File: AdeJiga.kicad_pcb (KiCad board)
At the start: 2 copper layers, 72 x 72 mm, 33 parts, among them J1 Screw_Terminal_01x03, J10 Conn_01x02_Pin, J11 Conn_01x02_Pin, J2 Screw_Terminal_01x02, J3 Screw_Terminal_01x03, J4 Conn_01x05_Pin, J5 Conn_01x02_Pin, J6 Conn_01x03_Pin, J7 Conn_01x02_Pin, J8 Conn_01x03_Pin, J9 Conn_01x04_Pin, K1 JJM1C_relay, K2 JJM1C_relay, M1 DC-DC-STEP-DOWN-LM2596, Q1 TIP127, Q3 TIP127, U2 ESP32-WROOM-32, U4 AMS1117

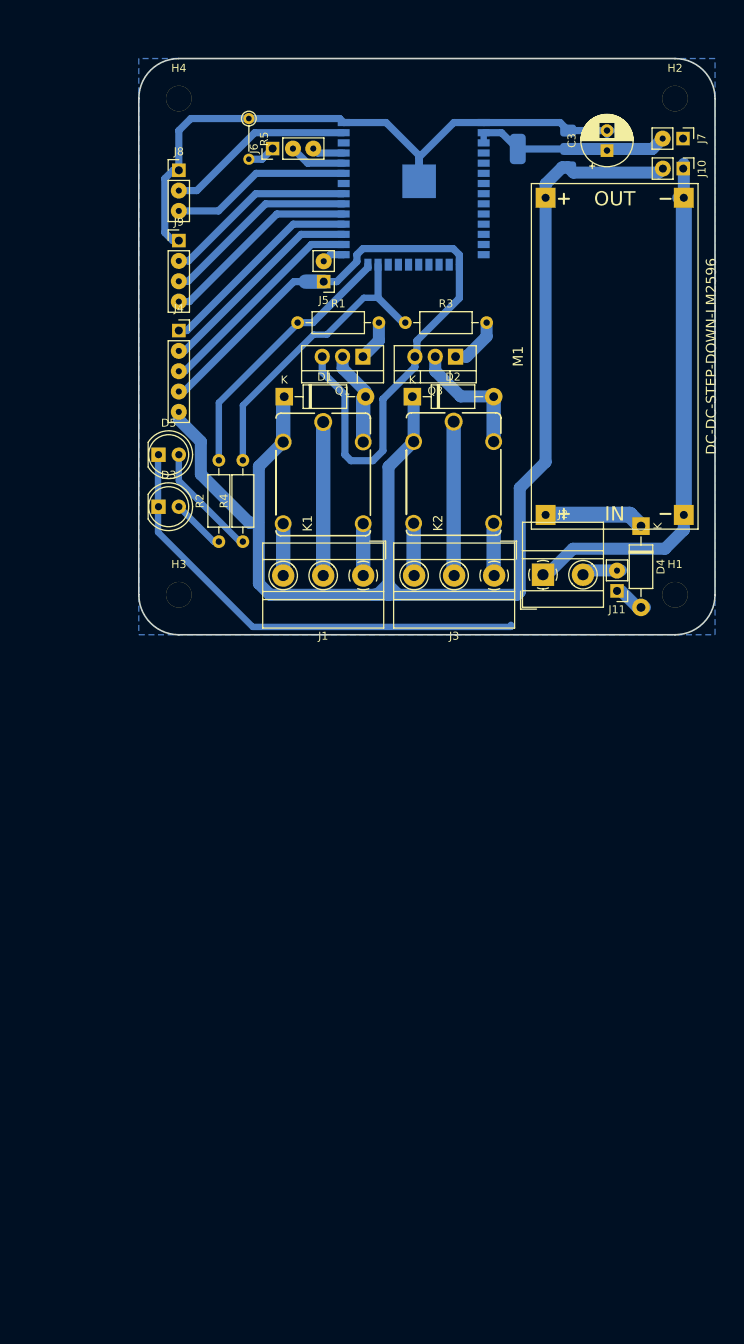
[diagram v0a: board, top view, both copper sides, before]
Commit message: 3 reles na jiga
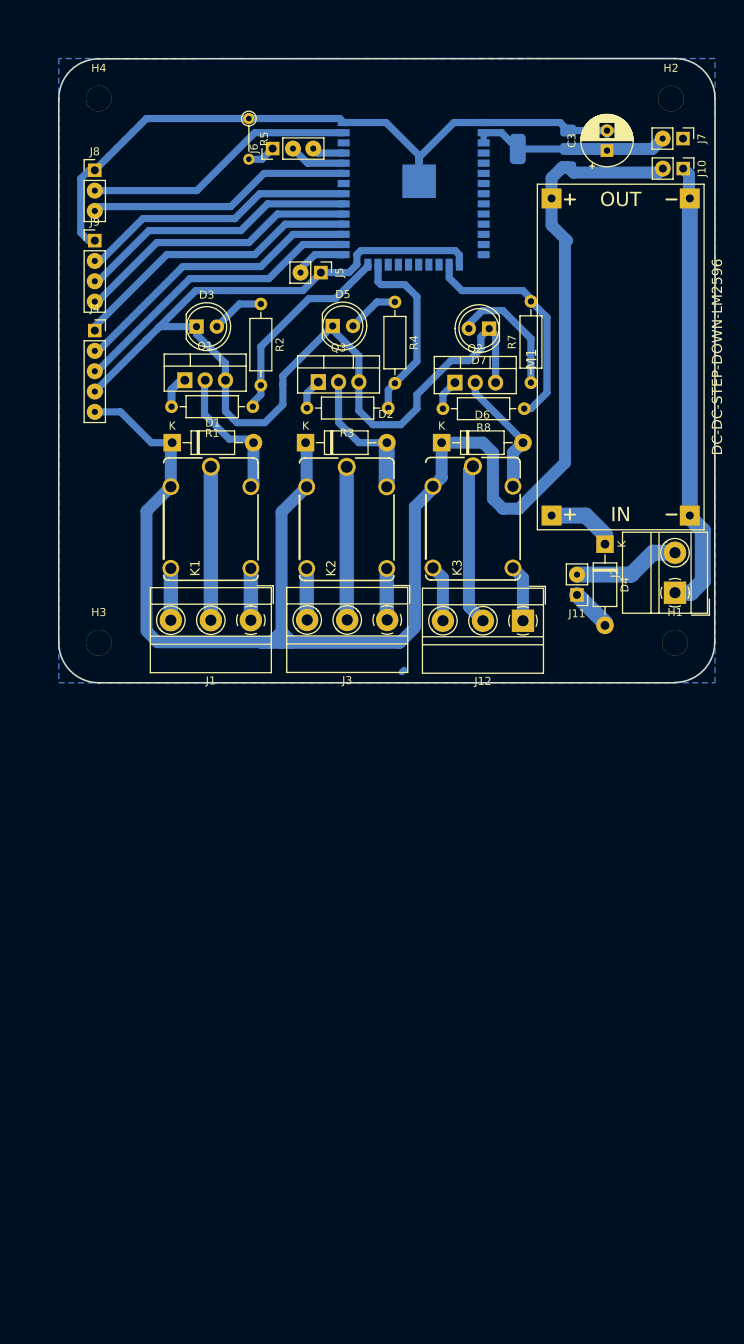
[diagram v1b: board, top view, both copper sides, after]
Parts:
- added D6: 1N4007, Diode_THT:D_DO-41_SOD81_P10.16mm_Horizontal, F.Cu at (159.8, 71.0)
- added D7: LED, LED_THT:LED_D5.0mm_Clear, F.Cu at (165.8, 56.8)
- added J12: Screw_Terminal_01x03, TerminalBlock_MetzConnect:TerminalBlock_MetzConnect_Type011_RT05503HBWC_1x03_P5.00mm_Horizontal, F.Cu at (170.0, 93.2)
- added K3: JJM1C_relay, Benzlab:JJM1C_relay, F.Cu at (163.8, 80.5)
- added Q2: TIP127, Package_TO_SOT_THT:TO-220-3_Vertical, F.Cu at (161.5, 63.5)
- added R7: 220, Resistor_THT:R_Axial_DIN0207_L6.3mm_D2.5mm_P10.16mm_Horizontal, F.Cu at (171.0, 63.5)
- added R8: 3.3k, Resistor_THT:R_Axial_DIN0207_L6.3mm_D2.5mm_P10.16mm_Horizontal, F.Cu at (170.2, 66.8)
- moved R4 35.5 mm to (154.0, 53.4), turned to -90 degrees
- moved R2 30.2 mm to (137.2, 53.7), turned to -90 degrees
- moved D5 27.1 mm to (146.2, 56.4)
- moved D3 23.0 mm to (129.2, 56.5)
- moved Q1 22.4 mm to (127.8, 63.2), turned to 0 degrees
- moved Q3 17.5 mm to (144.4, 63.4), turned to 0 degrees
- moved J2 16.7 mm to (189.0, 89.8), turned to 90 degrees
- moved D1 15.1 mm to (126.2, 71.0)
- moved J1 15.1 mm to (136.0, 93.2)
- moved K1 15.1 mm to (131.0, 80.5)
- moved D2 14.5 mm to (142.8, 71.0)
- moved K2 14.5 mm to (148.0, 80.6)
- moved J3 14.5 mm to (153.0, 93.2)
- moved R1 11.9 mm to (136.2, 66.5), turned to 180 degrees
- moved H3 11.7 mm to (117.0, 96.0)
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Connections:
- net GPIO16 renamed REL1
- net GPIO17 renamed REL2
- U2 pad 16: unconnected-(U2-IO13-Pad16) -> REL3
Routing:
- net REL3: track 0.00 -> 29.2 mm
- net +5V: track 175.3 -> 202.5 mm
- net Net-(J12-Pin_2): track 0.00 -> 20.2 mm
- net Net-(D7-A): track 0.00 -> 16.0 mm
- net Ativa_Relé_3: track 0.00 -> 15.9 mm
- net REL2: track 38.2 -> 23.2 mm
- net GND: track 297.3 -> 283.2 mm
- net GPIOC: track 26.1 -> 36.9 mm
- net GPIOE: track 24.6 -> 35.1 mm
- net GPIOA: track 27.2 -> 37.7 mm
- net GPIOG: track 23.6 -> 34.1 mm
- net GPIOD: track 25.1 -> 35.6 mm
- net GPIOB: track 26.6 -> 37.1 mm
- net GPIOH: track 22.5 -> 33.0 mm
- net GPIOF: track 24.1 -> 34.6 mm
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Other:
- board size 72 x 72 mm -> 82 x 78 mm

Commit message: Versão 3 consolidada, placa fabricada
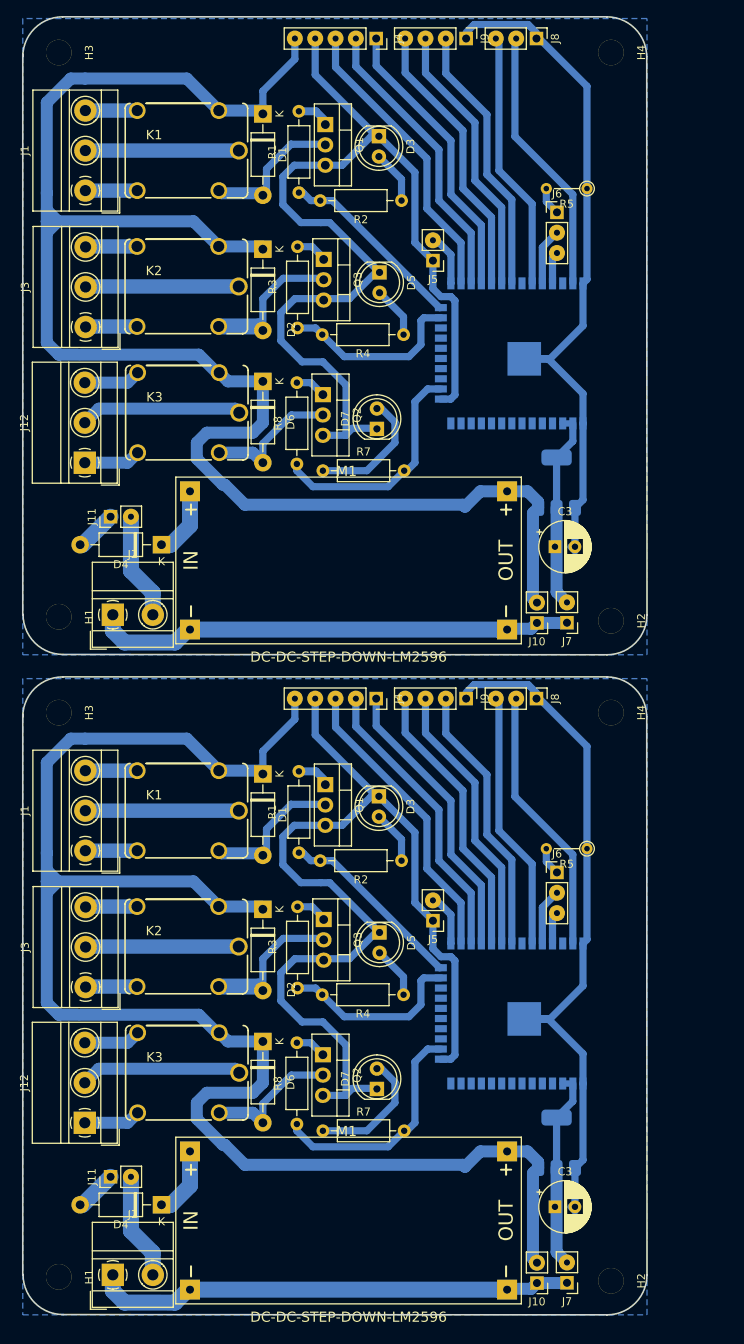
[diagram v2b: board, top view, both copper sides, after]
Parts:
- added C3: 220uF, Capacitor_THT:CP_Radial_D6.3mm_P2.50mm, F.Cu at (174.0, 166.5)
- added D1: 1N4007, Diode_THT:D_DO-41_SOD81_P10.16mm_Horizontal, F.Cu at (137.5, 112.4)
- added D2: 1N4007, Diode_THT:D_DO-41_SOD81_P10.16mm_Horizontal, F.Cu at (137.5, 129.3)
- added D3: LED, LED_THT:LED_D5.0mm_Clear, F.Cu at (152.0, 115.2)
- added D4: 1N4007, Diode_THT:D_DO-41_SOD81_P10.16mm_Horizontal, F.Cu at (124.8, 166.2)
- added D5: LED, LED_THT:LED_D5.0mm_Clear, F.Cu at (152.1, 132.2)
- added D6: 1N4007, Diode_THT:D_DO-41_SOD81_P10.16mm_Horizontal, F.Cu at (137.5, 145.8)
- added D7: LED, LED_THT:LED_D5.0mm_Clear, F.Cu at (151.8, 151.8)
- added H1: MountingHole, MountingHole:MountingHole_3.2mm_M3_DIN965, F.Cu at (112.0, 175.2)
- added H2: MountingHole, MountingHole:MountingHole_3.2mm_M3_DIN965, F.Cu at (181.0, 175.7)
- added H3: MountingHole, MountingHole:MountingHole_3.2mm_M3_DIN965, F.Cu at (112.0, 104.7)
- added H4: MountingHole, MountingHole:MountingHole_3.2mm_M3_DIN965, F.Cu at (181.0, 104.7)
- added J1: Screw_Terminal_01x03, TerminalBlock_MetzConnect:TerminalBlock_MetzConnect_Type011_RT05503HBWC_1x03_P5.00mm_Horizontal, F.Cu at (115.3, 122.0)
- added J10: Conn_01x02_Pin, Connector_PinHeader_2.54mm:PinHeader_1x02_P2.54mm_Vertical, F.Cu at (171.8, 176.0)
- added J11: Conn_01x02_Pin, Connector_PinHeader_2.54mm:PinHeader_1x02_P2.54mm_Vertical, F.Cu at (118.5, 162.7)
- added J12: Screw_Terminal_01x03, TerminalBlock_MetzConnect:TerminalBlock_MetzConnect_Type011_RT05503HBWC_1x03_P5.00mm_Horizontal, F.Cu at (115.2, 156.0)
- added J2: Screw_Terminal_01x02, TerminalBlock_MetzConnect:TerminalBlock_MetzConnect_Type011_RT05502HBWC_1x02_P5.00mm_Horizontal, F.Cu at (118.8, 175.0)
- added J3: Screw_Terminal_01x03, TerminalBlock_MetzConnect:TerminalBlock_MetzConnect_Type011_RT05503HBWC_1x03_P5.00mm_Horizontal, F.Cu at (115.3, 139.0)
- added J4: Conn_01x05_Pin, Connector_PinSocket_2.54mm:PinSocket_1x05_P2.54mm_Vertical, F.Cu at (151.7, 103.0)
- added J5: Conn_01x02_Pin, Connector_PinHeader_2.54mm:PinHeader_1x02_P2.54mm_Vertical, F.Cu at (158.8, 130.7)
- added J6: Conn_01x03_Pin, Connector_PinHeader_2.54mm:PinHeader_1x03_P2.54mm_Vertical, F.Cu at (174.2, 124.7)
- added J7: Conn_01x02_Pin, Connector_PinHeader_2.54mm:PinHeader_1x02_P2.54mm_Vertical, F.Cu at (175.5, 176.0)
- added J8: Conn_01x03_Pin, Connector_PinHeader_2.54mm:PinHeader_1x03_P2.54mm_Vertical, F.Cu at (171.7, 103.0)
- added J9: Conn_01x04_Pin, Connector_PinHeader_2.54mm:PinHeader_1x04_P2.54mm_Vertical, F.Cu at (162.9, 103.0)
- added K1: JJM1C_relay, Benzlab:JJM1C_relay, F.Cu at (128.0, 117.0)
- added K2: JJM1C_relay, Benzlab:JJM1C_relay, F.Cu at (127.9, 134.0)
- added K3: JJM1C_relay, Benzlab:JJM1C_relay, F.Cu at (128.0, 149.7)
- added M1: DC-DC-STEP-DOWN-LM2596, Benzlab:DC-DC-STEP-DOWN-LM2596, F.Cu at (148.2, 168.2)
- added Q1: TIP127, Package_TO_SOT_THT:TO-220-3_Vertical, F.Cu at (145.3, 113.7)
- added Q2: TIP127, Package_TO_SOT_THT:TO-220-3_Vertical, F.Cu at (145.0, 147.5)
- added Q3: TIP127, Package_TO_SOT_THT:TO-220-3_Vertical, F.Cu at (145.1, 130.6)
- added R1: 3.3k, Resistor_THT:R_Axial_DIN0207_L6.3mm_D2.5mm_P10.16mm_Horizontal, F.Cu at (142.0, 122.2)
- added R2: 220, Resistor_THT:R_Axial_DIN0207_L6.3mm_D2.5mm_P10.16mm_Horizontal, F.Cu at (154.8, 123.2)
- added R3: 3.3k, Resistor_THT:R_Axial_DIN0207_L6.3mm_D2.5mm_P10.16mm_Horizontal, F.Cu at (141.8, 139.2)
- added R4: 220, Resistor_THT:R_Axial_DIN0207_L6.3mm_D2.5mm_P10.16mm_Horizontal, F.Cu at (155.1, 140.0)
- added R5: 0, Resistor_THT:R_Axial_DIN0204_L3.6mm_D1.6mm_P5.08mm_Vertical, F.Cu at (178.0, 121.7)
- added R7: 220, Resistor_THT:R_Axial_DIN0207_L6.3mm_D2.5mm_P10.16mm_Horizontal, F.Cu at (145.0, 157.0)
- added R8: 3.3k, Resistor_THT:R_Axial_DIN0207_L6.3mm_D2.5mm_P10.16mm_Horizontal, F.Cu at (141.8, 156.1)
- added U2: ESP32-WROOM-32, RF_Module:ESP32-WROOM-32, B.Cu at (169.3, 142.3)
- added U4: AMS1117, Package_TO_SOT_SMD:SOT-223-3_TabPin2, B.Cu at (174.2, 158.5)
- moved H1 77.1 mm to (112.0, 92.8), turned to -90 degrees
- moved H3 73.9 mm to (112.0, 22.2), turned to -90 degrees
- moved J2 70.3 mm to (118.8, 92.5), turned to 0 degrees
- moved H2 65.7 mm to (181.0, 93.2), turned to -90 degrees
- moved H4 64.3 mm to (181.0, 22.2), turned to -90 degrees
- moved J7 62.2 mm to (175.5, 93.5), turned to 180 degrees
- moved J10 59.6 mm to (171.8, 93.5), turned to 180 degrees
- moved J11 59.1 mm to (118.5, 80.2), turned to 90 degrees
- moved J12 58.2 mm to (115.2, 73.5), turned to 90 degrees
- moved J8 57.6 mm to (171.7, 20.5), turned to -90 degrees
- moved J1 57.5 mm to (115.3, 39.5), turned to 90 degrees
- moved D4 55.4 mm to (124.8, 83.8), turned to 180 degrees
- moved J9 52.8 mm to (162.9, 20.5), turned to -90 degrees
- moved J3 52.5 mm to (115.3, 56.5), turned to 90 degrees
- moved J4 50.7 mm to (151.7, 20.5), turned to -90 degrees
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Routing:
- net GND: track 283.2 -> 554.3 mm
- net +5V: track 202.5 -> 416.6 mm
- net GPIOA: track 37.7 -> 74.2 mm
- net GPIOB: track 37.1 -> 73.1 mm
- net GPIOC: track 36.9 -> 72.1 mm
- net GPIOD: track 35.6 -> 70.1 mm
- net GPIOE: track 35.1 -> 69.1 mm
- net GPIOF: track 34.6 -> 68.0 mm
- net GPIOG: track 34.1 -> 67.3 mm
- net GPIOH: track 33.0 -> 65.0 mm
- net REL3: track 29.2 -> 58.4 mm
- net +3.3V: track 25.0 -> 50.0 mm
- net REL2: track 23.2 -> 46.3 mm
- net REL1: track 25.6 -> 47.4 mm
- net Net-(J12-Pin_2): track 20.2 -> 40.5 mm
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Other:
- board size 82 x 78 mm -> 78 x 162.2 mm
- board text removed: "-"
- board text removed: "3V3"
- board text removed: "5V"
- board text removed: "A"
- board text removed: "B"
- board text removed: "C"
- board text removed: "D"
- board text removed: "E"
- board text removed: "F"
- board text removed: "G"
- board text removed: "H"
- board text removed: "NA"
- board text removed: "NF"
